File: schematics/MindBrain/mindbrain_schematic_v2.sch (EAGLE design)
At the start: 51 parts, among them CON1 POWER, IC1 TL084, IC2 TL084

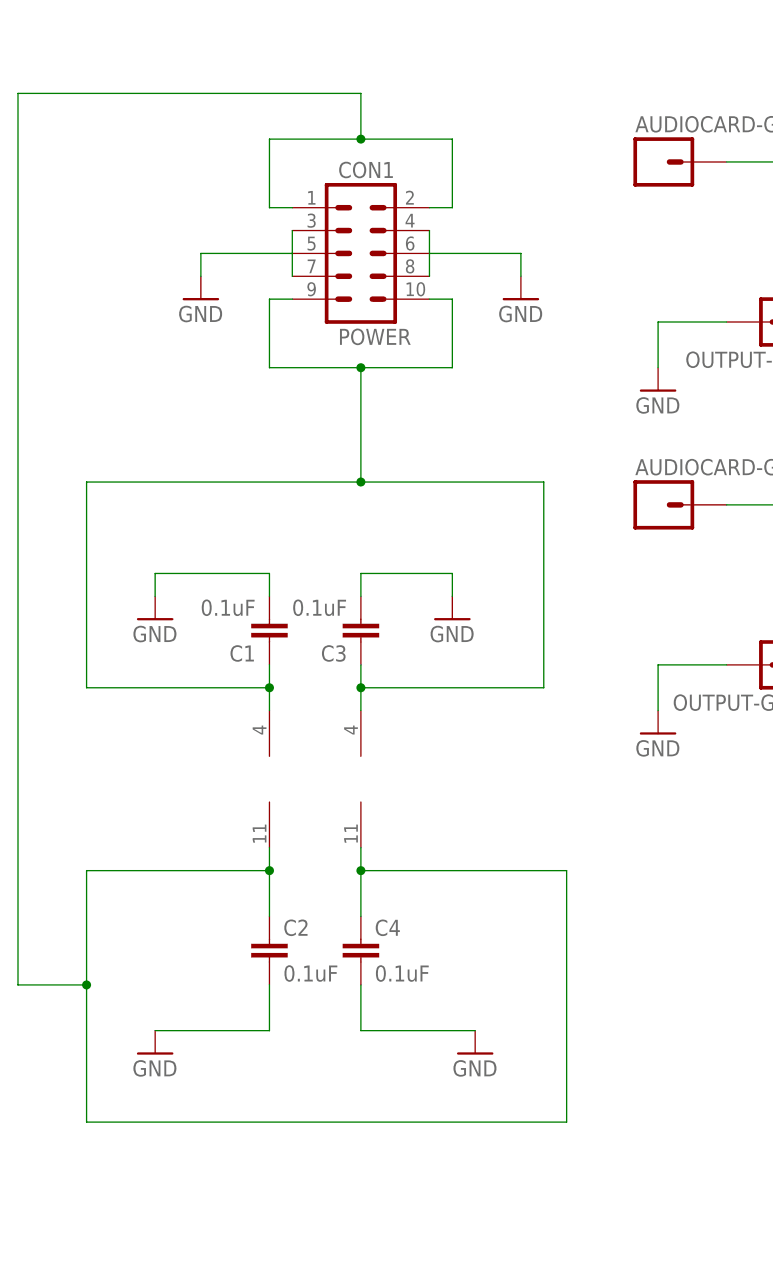
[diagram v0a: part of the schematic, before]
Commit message: cleaned up schematic thx nathan
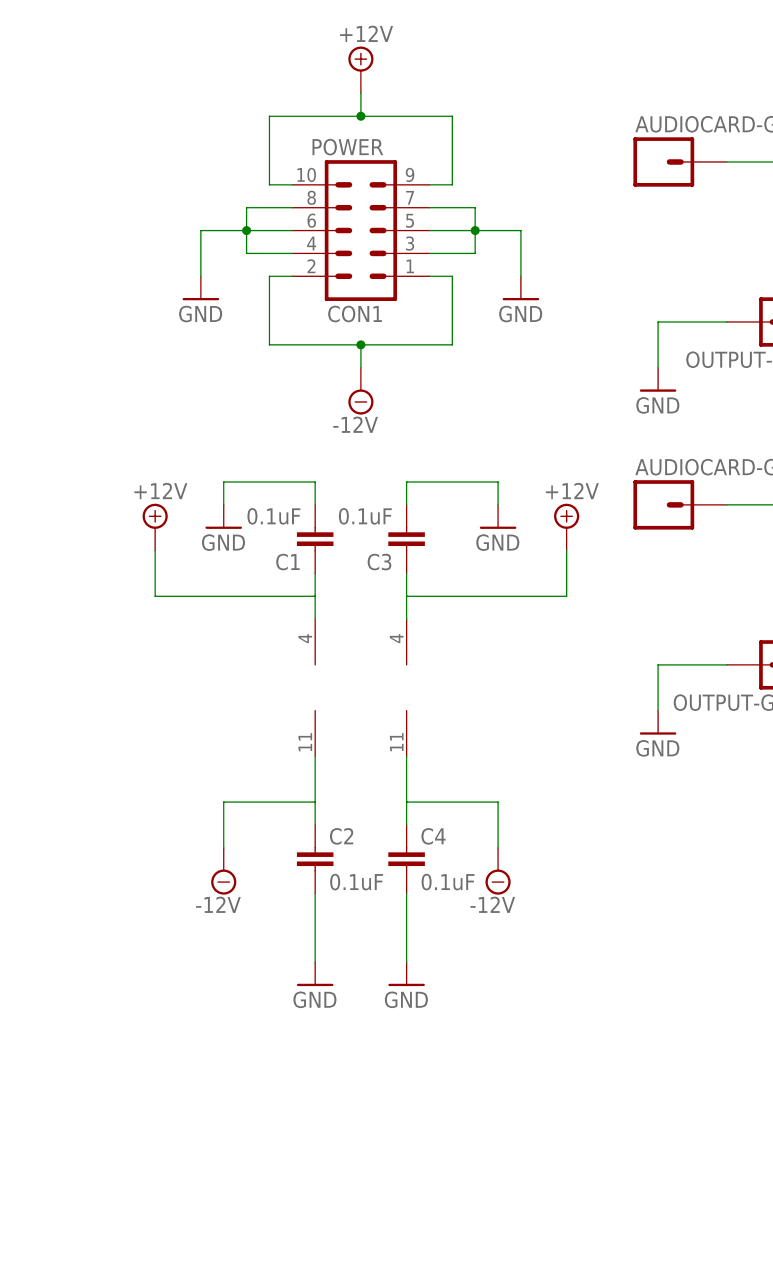
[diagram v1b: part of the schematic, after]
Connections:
- net N$25 renamed +12V
- net N$27 renamed -12V
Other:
- moved on the sheet: C1, C2, C3, C4, CON1
